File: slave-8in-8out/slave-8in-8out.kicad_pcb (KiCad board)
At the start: 2 copper layers, 61 x 72.4 mm, 87 parts, among them J1 Conn_01x06_Male, J2 Screw_Terminal_01x02, J3 Conn_01x06_Female, J4 Screw_Terminal_01x04, J5 Screw_Terminal_01x04, J6 Screw_Terminal_01x04, J7 Screw_Terminal_01x04, J8 Conn_01x10_Male, J9 Screw_Terminal_01x02, SW1 SW_DIP_x05, U1 MCP23017_SO, U10 ULN2803A, U2 EL817, U3 EL817, U4 EL817, U5 EL817, U6 EL817, U7 EL817, U8 EL817, U9 EL817

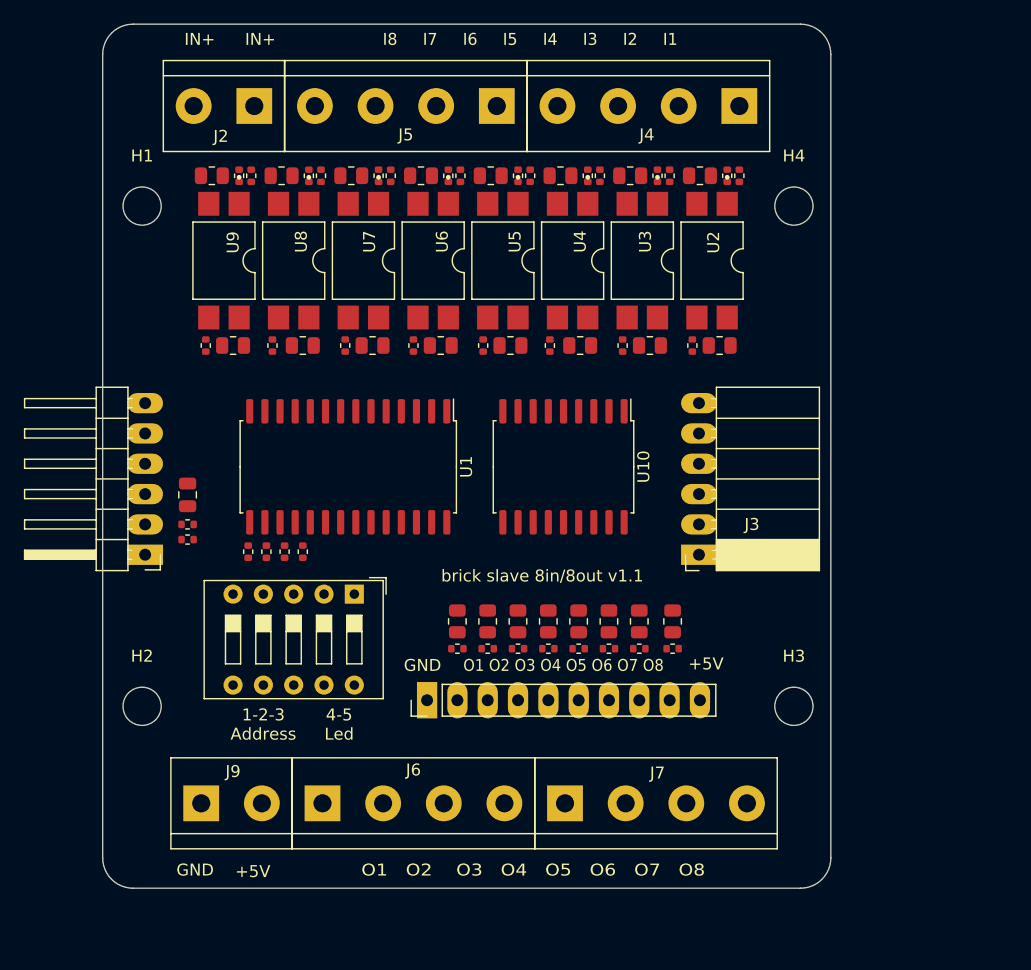
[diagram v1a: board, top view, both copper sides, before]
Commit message: slave-8in-8out-0.1
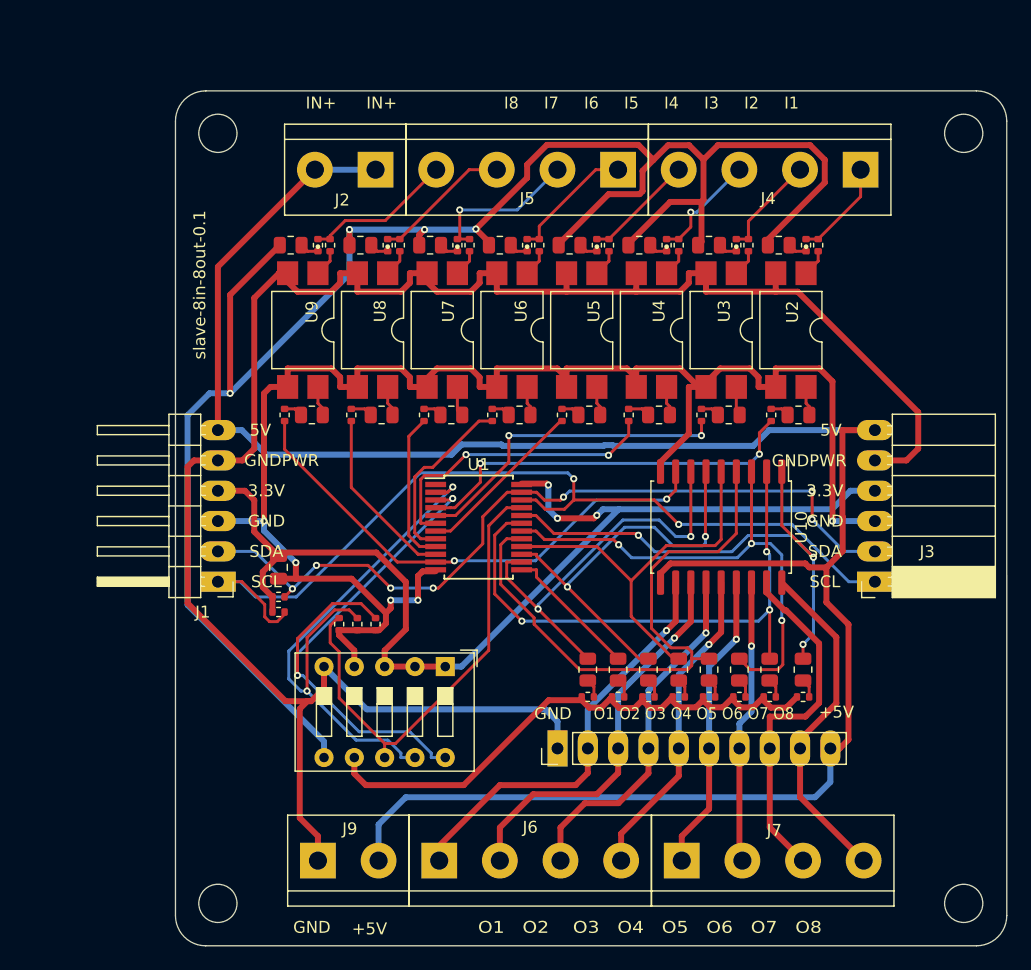
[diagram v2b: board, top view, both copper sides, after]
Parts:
- removed R11: 10k, Resistor_SMD:R_0402_1005Metric
- U1: value MCP23017_SO -> PCF8575; footprint Package_SO:SOIC-28W_7.5x17.9mm_P1.27mm -> Package_SO:SSOP-24_5.3x8.2mm_P0.65mm
- moved H2 83.9 mm to (135.6, 63.8)
- moved H4 60.1 mm to (135.6, 128.3)
- moved H3 51.0 mm to (73.2, 128.3)
- moved J3 14.9 mm to (128.2, 101.3)
- moved U10 14.1 mm to (115.3, 96.7)
- moved U1 12.0 mm to (95.0, 96.7), turned to 0 degrees
- moved D1 11.6 mm to (122.2, 108.7)
- moved D3 11.6 mm to (116.8, 108.7)
- moved D5 11.6 mm to (111.8, 108.7)
- moved D7 11.6 mm to (104.1, 108.7)
- moved D8 11.6 mm to (106.7, 108.7)
- moved J8 11.6 mm to (101.6, 115.3)
- moved R47 11.6 mm to (122.2, 111.0)
- moved R48 11.6 mm to (119.4, 111.0)
- moved R50 11.6 mm to (114.3, 111.0)
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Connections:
- D7 pad 2: GPB7 -> GPA1
- D8 pad 2: GPA1 -> GPA0
- R46 pad 1: GPA0 -> GPB7
- U1 pad 1: GPB0 -> unconnected-(U1-Pad1)
- U1 pad 10: GND -> GPB6
- U1 pad 11: unconnected-(U1-Pad11) -> GPB7
- U1 pad 12: SCL -> GND
- U1 pad 13: SDA -> GPA0
- U1 pad 14: unconnected-(U1-Pad14) -> GPA1
- U1 pad 15: A0 -> GPA2
- U1 pad 16: A1 -> GPA3
- U1 pad 17: A2 -> GPA4
- U1 pad 18: Net-(R11-Pad1) -> GPA5
- U1 pad 19: unconnected-(U1-Pad19) -> GPA6
- U1 pad 2: GPB1 -> A1
- U1 pad 20: unconnected-(U1-Pad20) -> GPA7
- U1 pad 21: GPA0 -> A0
- U1 pad 22: GPA1 -> SCL
- U1 pad 23: GPA2 -> SDA
- U1 pad 24: GPA3 -> +3V3
- U1 pad 3: GPB2 -> A2
- U1 pad 4: GPB3 -> GPB0
- U1 pad 5: GPB4 -> GPB1
- U1 pad 6: GPB5 -> GPB2
- U1 pad 7: GPB6 -> GPB3
- U1 pad 8: GPB7 -> GPB4
- U1 pad 9: +3V3 -> GPB5
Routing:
- net +5V: track 0.00 -> 179.3 mm
- net GNDPWR: track 0.00 -> 169.6 mm
- net LED_GNDPWR: track 0.00 -> 156.4 mm, vias 0 -> 4
- net GND: track 0.00 -> 136.3 mm, vias 0 -> 5
- net +3V3: track 0.00 -> 92.1 mm, vias 0 -> 3
- net SCL: track 0.00 -> 77.7 mm, vias 0 -> 2
- net SDA: track 0.00 -> 67.6 mm, vias 0 -> 7
- net GPA4: track 0.00 -> 50.0 mm
- net A2: track 0.00 -> 48.5 mm, vias 0 -> 2
- net LED_GND: track 0.00 -> 47.8 mm
- net GPA6: track 0.00 -> 47.7 mm, vias 0 -> 3
- net A1: track 0.00 -> 46.8 mm, vias 0 -> 2
- net GPA7: track 0.00 -> 44.2 mm, vias 0 -> 3
- net GPB7: track 0.00 -> 43.1 mm, vias 0 -> 2
- net GPA5: track 0.00 -> 43.1 mm, vias 0 -> 3
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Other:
- board size 61 x 72.4 mm -> 69.6 x 71.6 mm
- board text added: "3.3V"
- board text added: "5V"
- board text added: "GNDPWR"
- board text added: "SCL"
- board text added: "SDA"
- board text added: "slave-8in-8out-0.1"
- board text removed: "1-2-3 Address"
- board text removed: "4-5 Led"
- board text removed: "brick slave 8in/8out v1.1"
